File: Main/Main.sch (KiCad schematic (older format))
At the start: 63 parts, among them J1 Power, J2 ModeSW, J3 SGND, J4 -5V, J5 MA1M→, J6 LFO_out, J7 →MA1M, U1 LA6358-2, U2 NE556, U3 NJM4556-1, U4 MCP6002

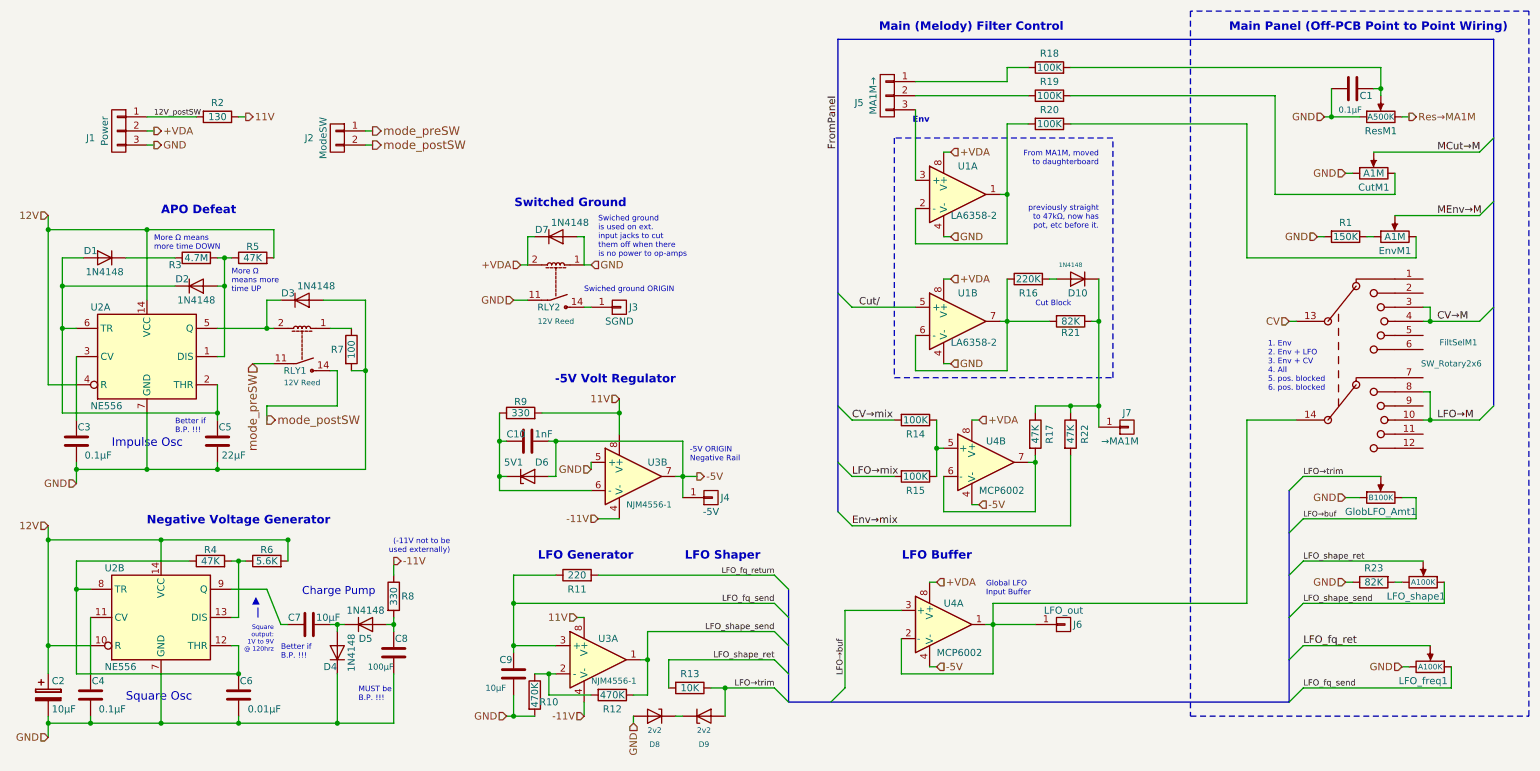
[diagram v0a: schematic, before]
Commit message: update LFO design
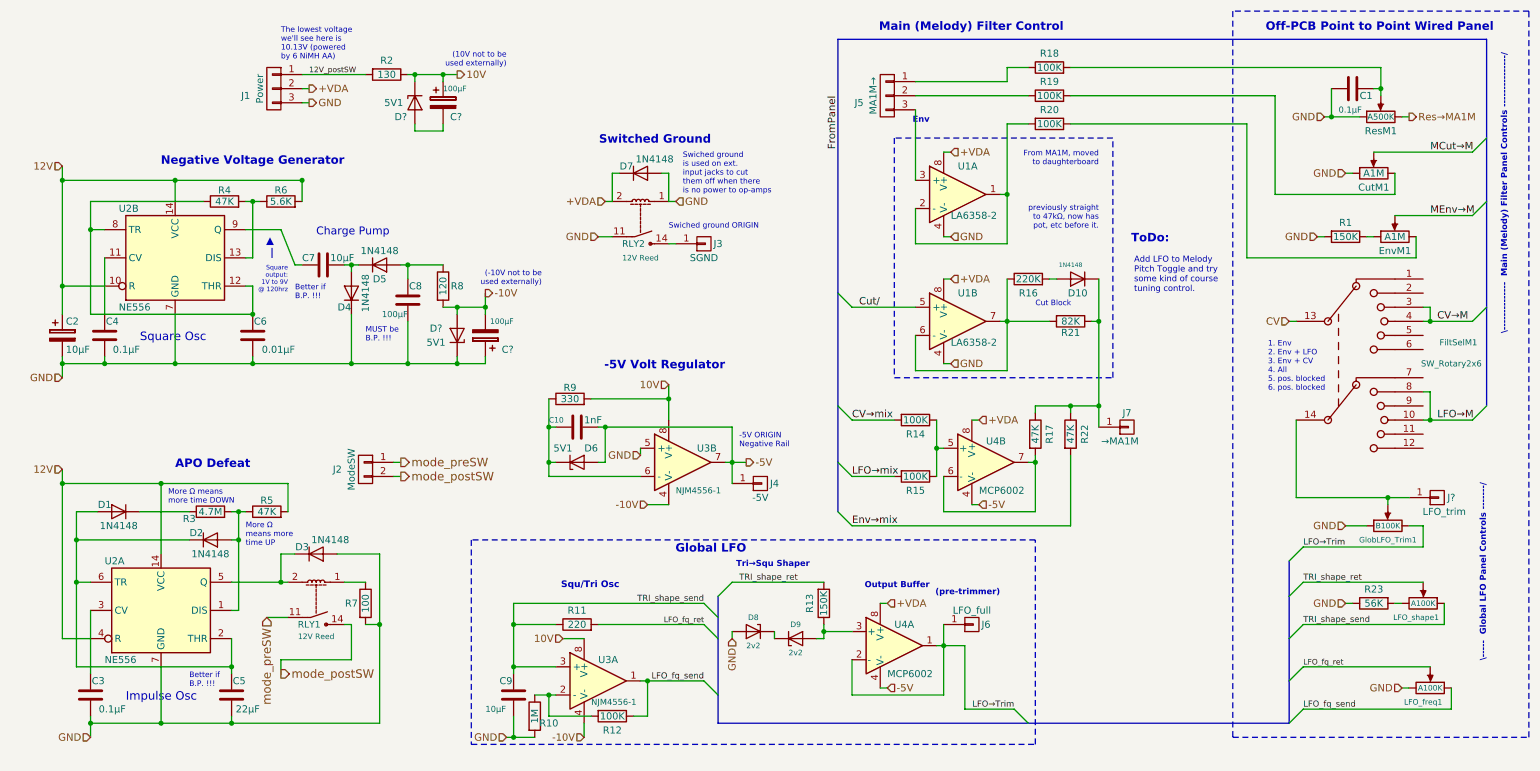
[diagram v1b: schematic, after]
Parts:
- added C? (x2): 100µF, symbol CP
- added D? (x2): 5V1, symbol D_Zener
- added J?: LFO_trim, symbol CONN_01X01
- J6: value LFO_out -> LFO_full
- R10: value 470K -> 1M
- R12: value 470K -> 100K
- R13: value 10K -> 150K
- R23: value 82K -> 56K
- R8: value 330 -> 120
- renumbered GlobLFO_Amt1 to GlobLFO_Trim1
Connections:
- net LFO_fq_return is gone; now on net LFO_fq_ret: R11.2
- net GND: now also C?.1, D?.1 (K)
- net LFO_fq_send: now also R12.1, U3.1; no longer C9.1, R11.1, U3.3 (+)
- net LFO→Trim: now reaches J6.1 (P1), U4.1, U4.2 (-)
- net LFO→Trim: now also GlobLFO_Trim1.3; no longer FiltSelM1.14
- net at C8.1, D5.2 (A): now also R8.1; no longer R8.2
- net -11V renamed -10V
- net -10V: now also R8.2, C?.2, D?.2 (A); no longer R8.1
- net 11V renamed 10V
- net 10V: now also C?.1, D?.1 (K)
- net LFO_shape_ret renamed TRI_shape_ret
- removed net LFO_shape_send: LFO_shape1.1, R12.1, U3.1
- net LFO→buf: no longer names the net of U4.3 (+)
- net LFO→buf: now also D9.2 (A), R13.1; no longer GlobLFO_Trim1.3
- removed net LFO→trim: D9.2 (A), GlobLFO_Trim1.2, R13.1
- new net: FiltSelM1.14, GlobLFO_Trim1.2, J?.1 (P1)
- new net: C?.2, D?.2 (A)
- new net TRI_shape_send: C9.1, LFO_shape1.1, R11.1, U3.3 (+)
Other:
- note added: "(-10V not to be \nused externally)"
- note added: "(10V not to be \nused externally)"
- note added: "(pre-trimmer)"
- note added: "Add LFO to Melody\nPitch Toggle and try\nsome kind of course\ntuning control."
- note added: "Global LFO"
- note added: "Off-PCB Point to Point Wired Panel"
- note added: "Output Buffer"
- note added: "Squ/Tri Osc"
- note added: "The lowest voltage\nwe'll see here is \n10.13V (powered\nby 6 NiMH AA)"
- note added: "ToDo:"
- note added: "Tri→Squ Shaper"
- note added: "\----- Global LFO Panel Controls -------/"
- note added: "\-------------- Main (Melody) Filter Panel Controls ---------------/"
- note removed: "(-11V not to be \nused externally)"
- note removed: "Global LFO \nInput Buffer"
- note removed: "LFO Buffer"
- note removed: "LFO Generator"
- note removed: "LFO Shaper"
- note removed: "Main Panel (Off-PCB Point to Point Wiring)"
- moved on the sheet: C10, C2, C3, C4, C5, C6, C7, C8, C9, D1, D2, D3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
